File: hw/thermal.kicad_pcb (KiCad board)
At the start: 2 copper layers, 110 x 60 mm, 40 parts, among them IC1 ATTINY2313-P, J1 USB_2, J2 RJ12, J3 DB9, J4 JACK_2P, Q1 IRL530N, Q2 IRL530N, U1 LM7805, U2 LTV847, X1 12MHz

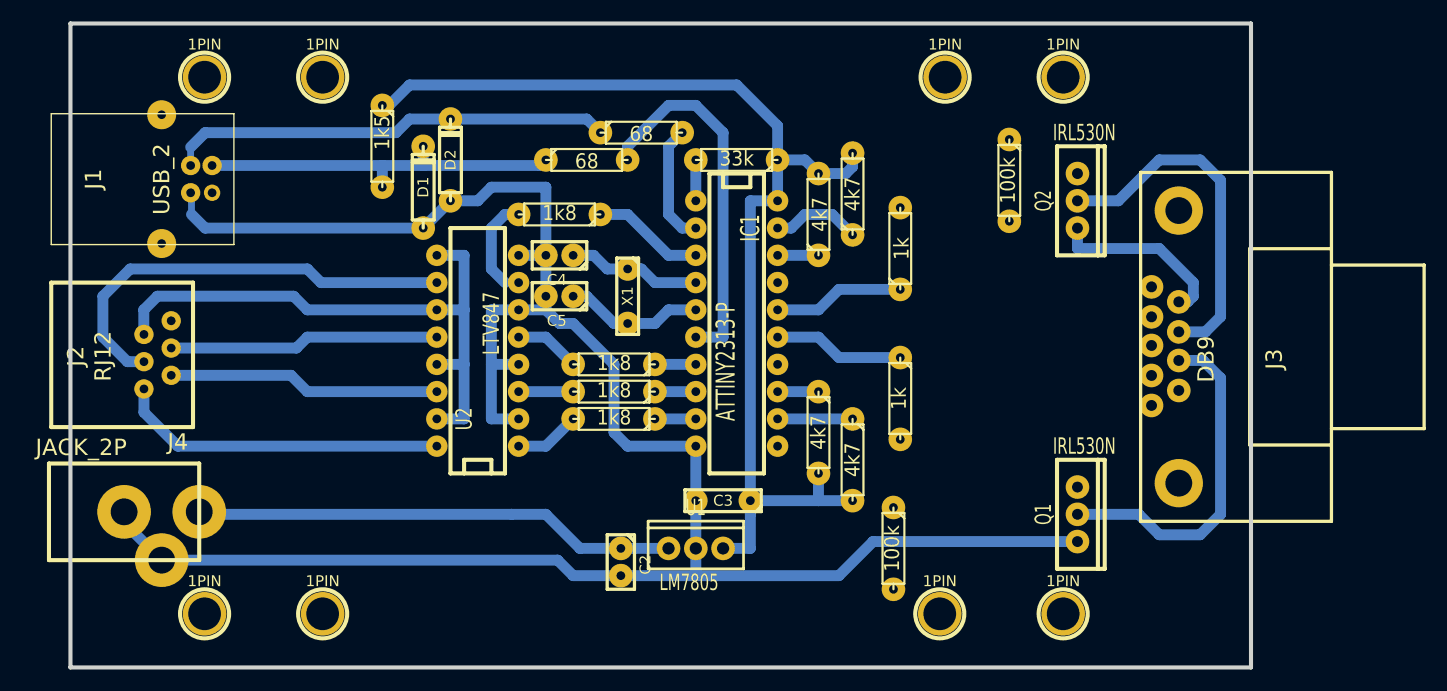
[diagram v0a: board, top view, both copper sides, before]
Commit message: V2 hardware schematics and pcb
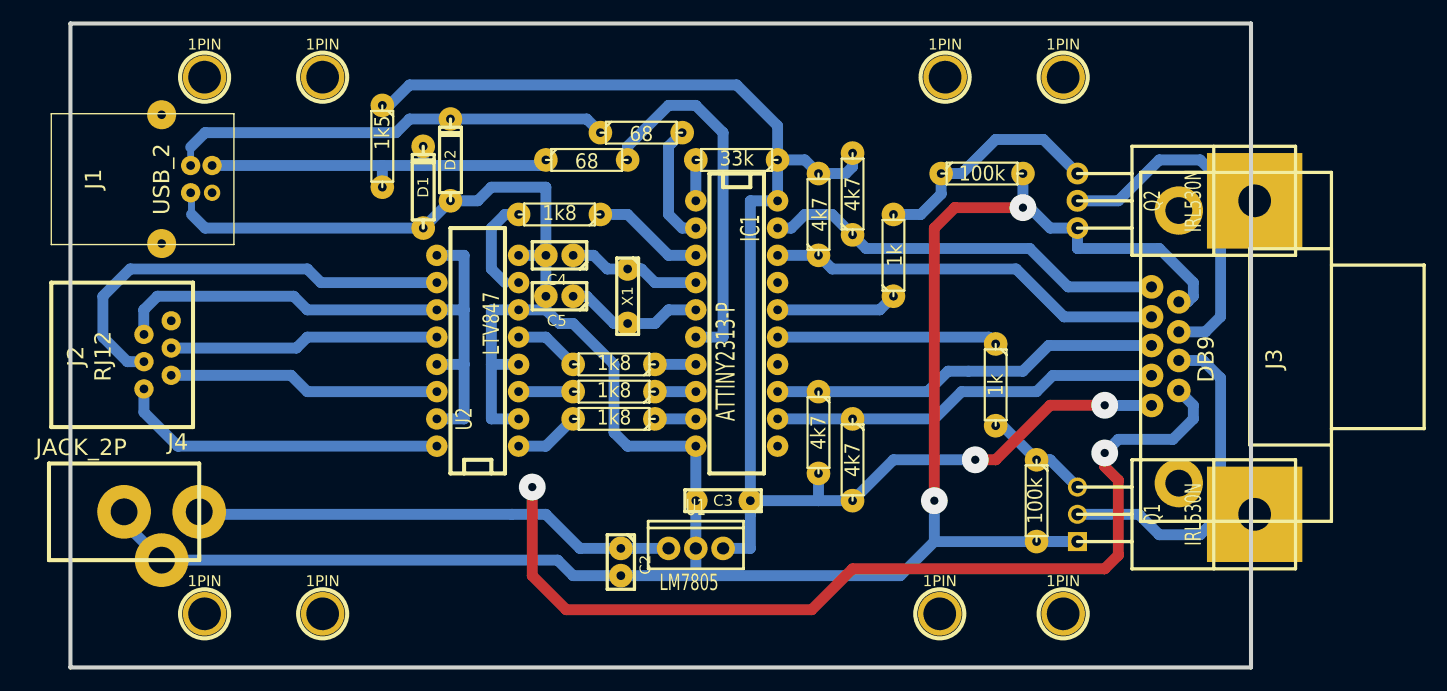
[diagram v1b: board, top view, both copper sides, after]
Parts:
- Q1, Q2: footprint TO220_VERT -> TO220GDS
- moved R15 14.1 mm to (160.0, 124.5)
- moved R13 8.98 mm to (156.2, 113.7)
- moved R16 2.62 mm to (154.9, 94.0), turned to 0 degrees
- moved R14 0.90 mm to (146.7, 101.6)
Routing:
- net +12V: track 45.1 -> 136.8 mm, vias 0 -> 2
- net GND: track 216.5 -> 267.6 mm, vias 0 -> 2
- net /TEMP2: track 3.81 -> 37.2 mm
- net /TEMP3: track 3.81 -> 36.6 mm
- net VCC: track 104.8 -> 136.3 mm, vias 0 -> 2
- net /TEMP1: track 8.30 -> 38.2 mm
- net /TEMP4: track 6.99 -> 36.5 mm
- net N-0000024: track 0.00 -> 22.5 mm
- net N-0000023: track 0.00 -> 9.99 mm
- net /FAN1: track 12.2 -> 20.6 mm
- net /FAN2: track 12.2 -> 11.3 mm
